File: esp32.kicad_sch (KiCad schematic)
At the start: 45 parts, among them SW2 BOOT, U6 ESP32-S3R8, U7 W25Q128JVSIQ, Y1 40MHz

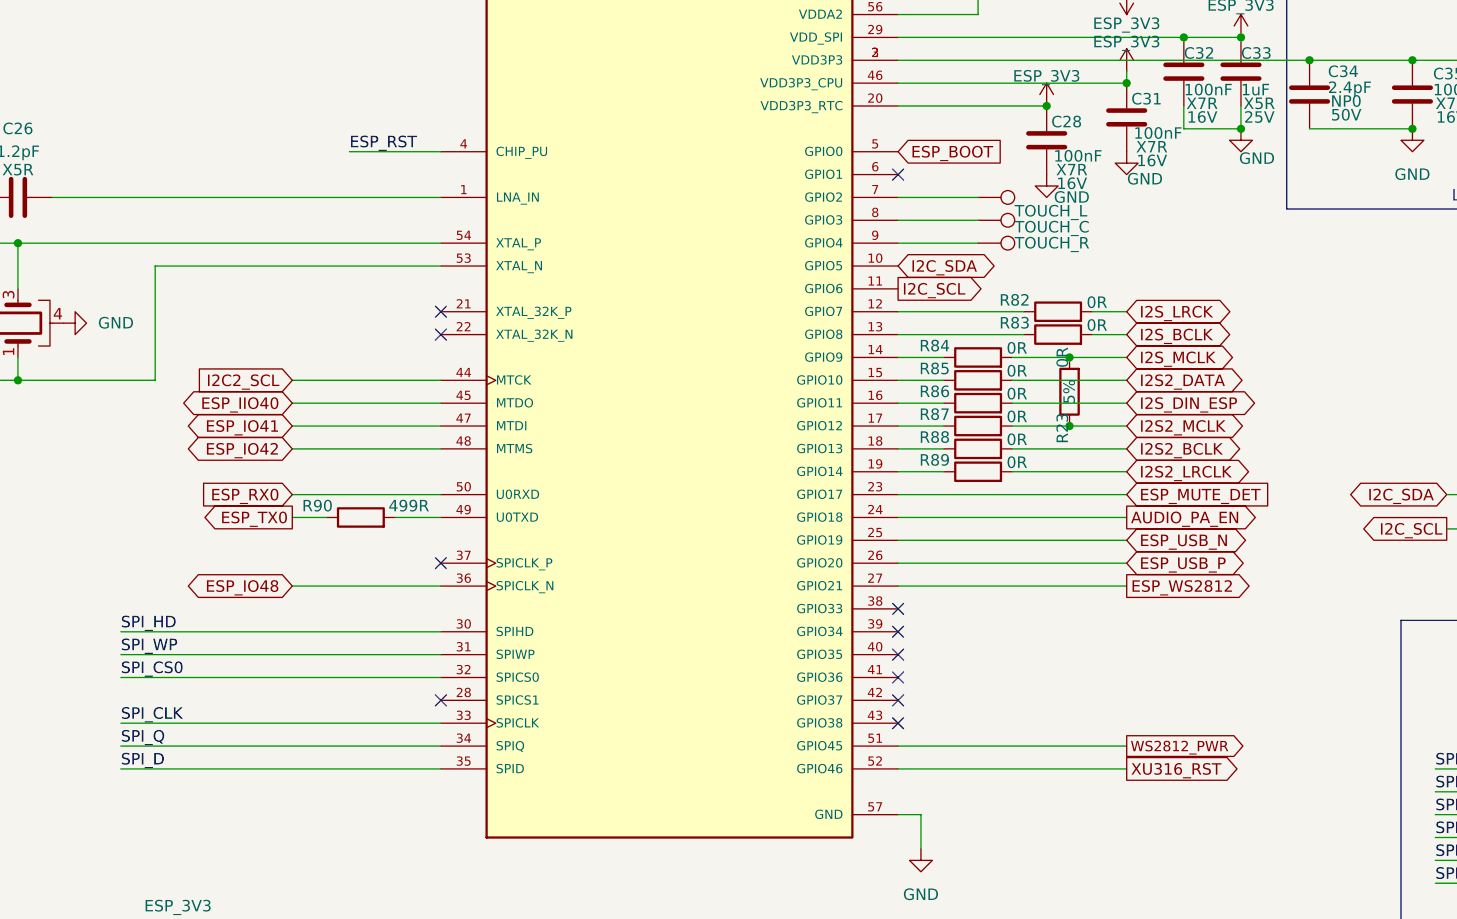
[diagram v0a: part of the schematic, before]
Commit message: routing done
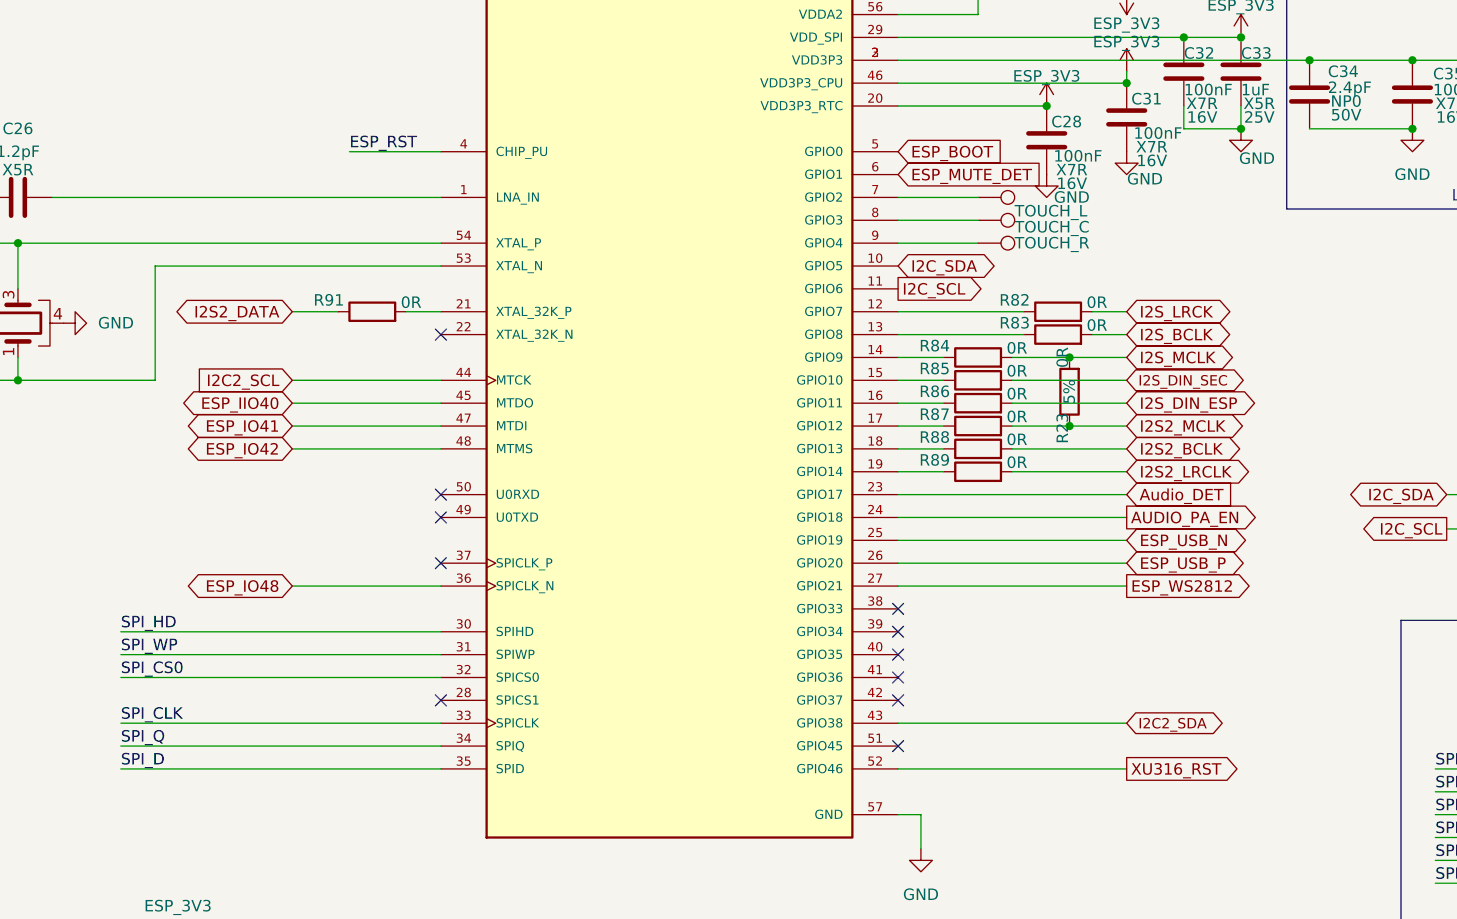
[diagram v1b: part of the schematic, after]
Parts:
- removed R90: 499R, Resistor_SMD:R_0402_1005Metric, symbol Device:R
- added R91: 0R, Resistor_SMD:R_0402_1005Metric, symbol Device:R
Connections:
- net ESP_MUTE_DET: now also U6.6 (GPIO1); no longer U6.23 (GPIO17)
- net I2S2_DATA: now also R91.1; no longer R85.2
- net at U6.21 (XTAL_32K_P): now also R91.2
- net I2C2_SDA: now reaches U6.43 (GPIO38)
- net ESP_RX0: no longer names the net of U6.50 (U0RXD)
- net WS2812_PWR: no longer names the net of U6.51 (GPIO45)
- new net Audio_DET: U6.23 (GPIO17)
- new net I2S_DIN_SEC: R85.2

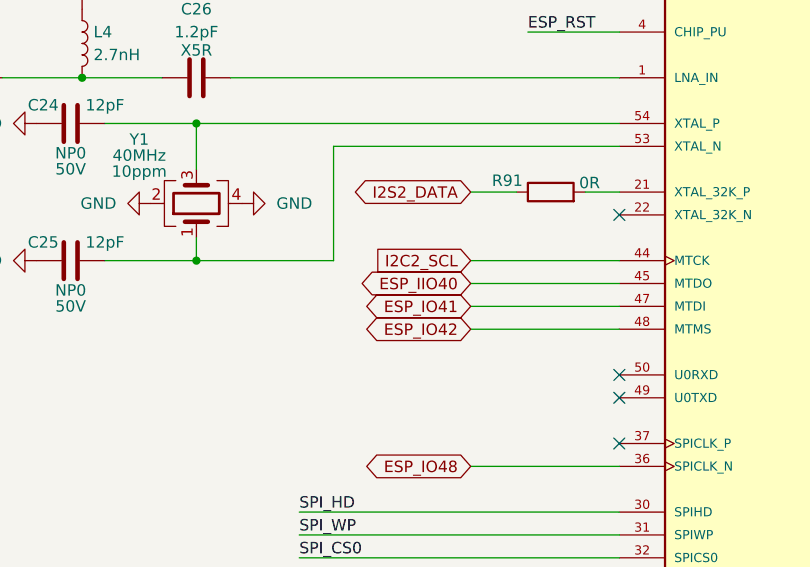
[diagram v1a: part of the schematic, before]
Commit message: routing done
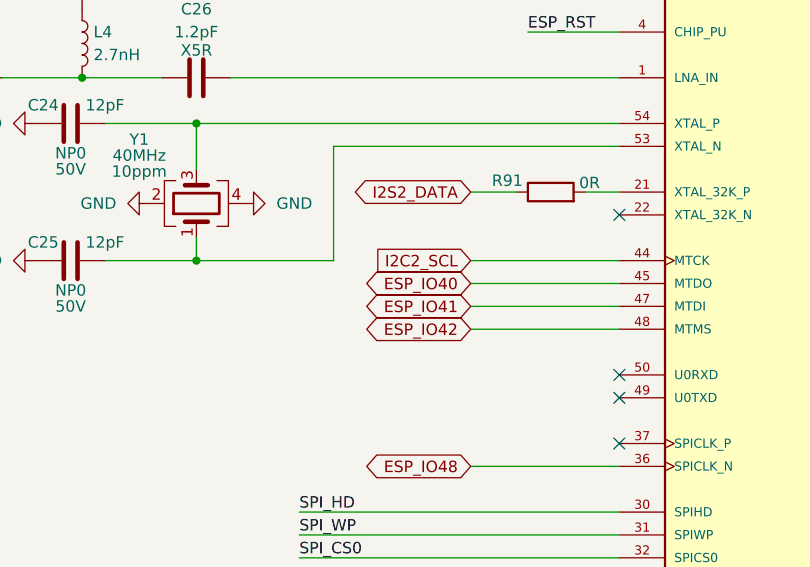
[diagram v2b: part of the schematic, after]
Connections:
- net ESP_IIO40 renamed ESP_IO40
